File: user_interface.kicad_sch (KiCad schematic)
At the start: 29 parts, among them J3 Внутр. коннектор потенциометр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, J4 Внутр. коннектор галлетника (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, SW1 Кнопка тактовая 6x6 без фикса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, SW2 Кнопка тактовая 6x6 без фикса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, SW3 Кнопка тактовая 6x6 без фикса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, SW4 Кнопка тактовая 6x6 без фикса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, SW5 Кнопка тактовая 6x6 без фикса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, SW6 Кнопка тактовая 6x6 без фикса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

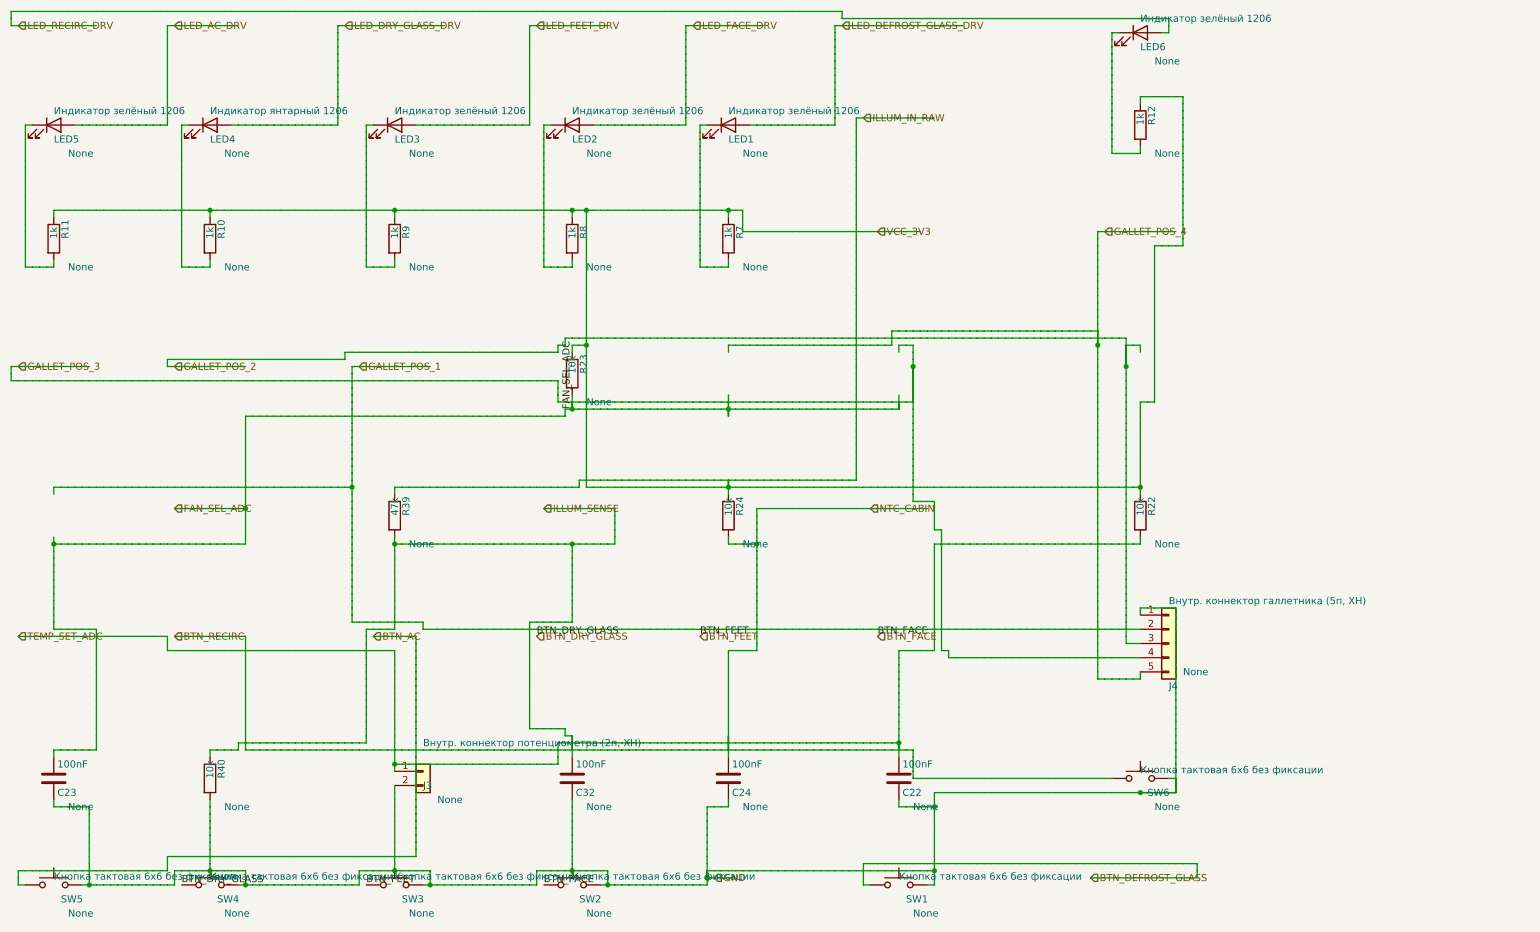
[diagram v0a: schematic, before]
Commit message: fix writer
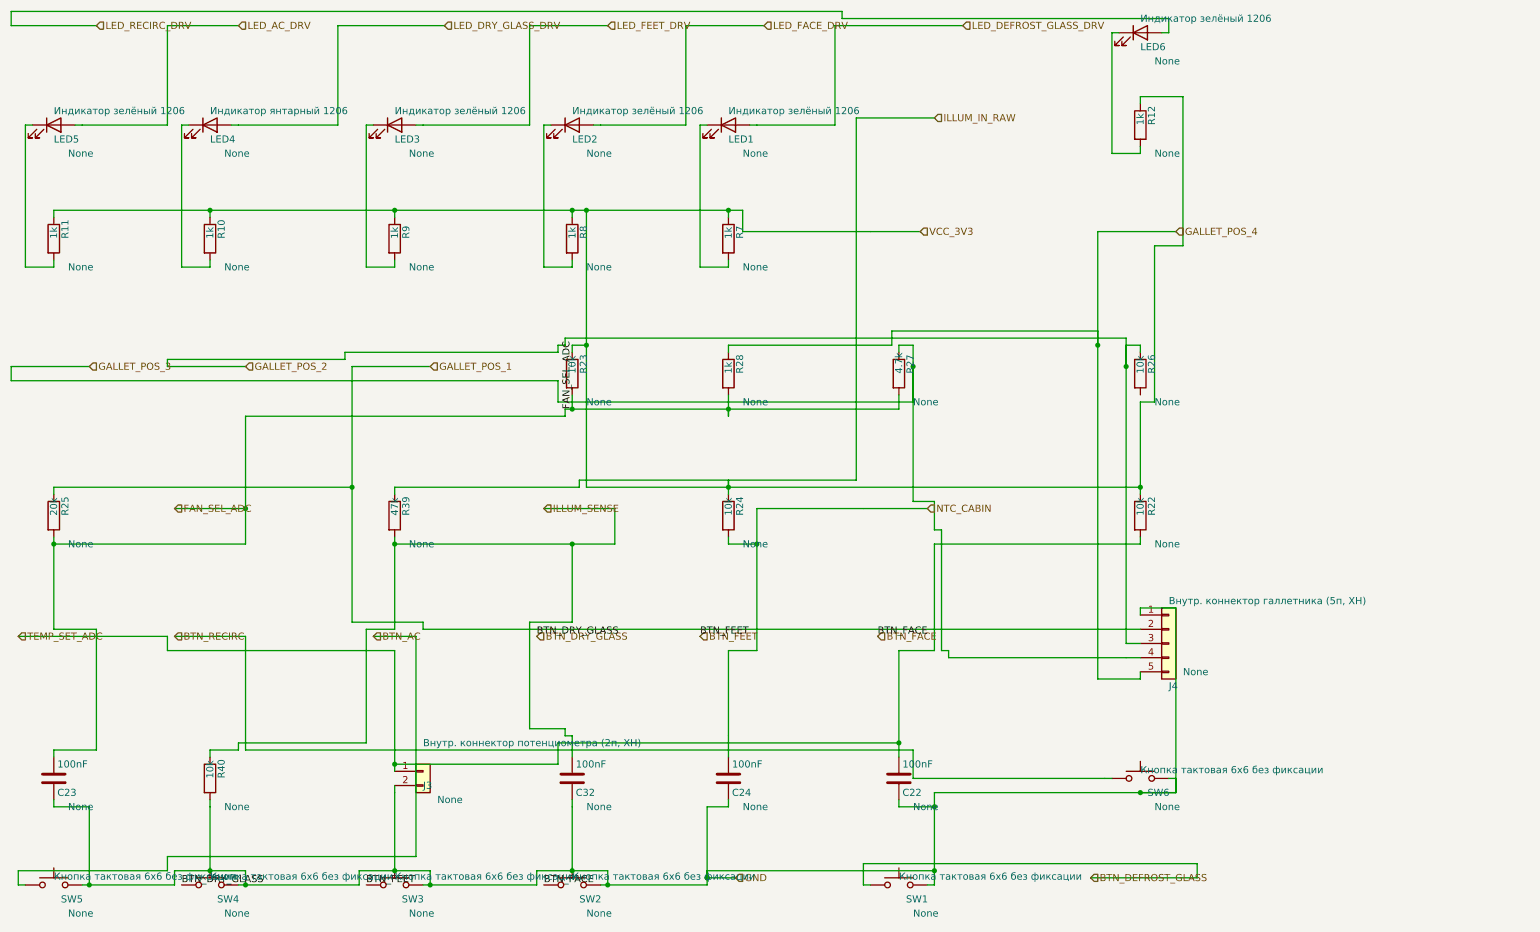
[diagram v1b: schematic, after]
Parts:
- added R25: 20k, symbol Device:R
- added R26: 10k, symbol Device:R
- added R27: 4.7k, symbol Device:R
- added R28: 1k, symbol Device:R
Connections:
- net BTN_AC: no longer C22.1, C22.2, C23.1, C23.2, C24.1, C24.2, C32.1, C32.2, J3.1 (Pin_1), J3.2 (Pin_2), J4.1 (Pin_1), J4.2 (Pin_2), J4.3 (Pin_3), J4.4 (Pin_4), J4.5 (Pin_5), LED1.1 (K), LED2.1 (K), LED3.1 (K), LED4.1 (K), R10.1, R10.2, R11.1, R12.1, R22.1, R22.2, R23.1, R23.2, R24.1, R24.2, R39.1, R39.2, R40.1, R40.2, R7.1, R7.2, R8.1, R8.2, R9.1, R9.2, SW1.1, SW1.2, SW2.2, SW3.2, SW4.2, SW5.2, SW6.1, SW6.2
- new net: LED3.1 (K), R9.2
- new net: LED1.1 (K), R7.2
- new net: LED2.1 (K), R8.2
- new net: LED4.1 (K), R10.2
- new net BTN_DEFROST_GLASS: SW1.1
- new net BTN_RECIRC: SW6.1
- new net FAN_SEL_ADC: C23.1, R23.2, R25.2, R27.2, R28.2
- new net GALLET_POS_1: J4.2 (Pin_2), R25.1
- new net GALLET_POS_2: J4.3 (Pin_3), R26.1
- new net GALLET_POS_3: J4.4 (Pin_4), R27.1
- new net GALLET_POS_4: J4.5 (Pin_5), R28.1
- new net GND: C22.2, C23.2, C24.2, C32.2, J3.2 (Pin_2), J4.1 (Pin_1), R40.2, SW1.2, SW2.2, SW3.2, SW4.2, SW5.2, SW6.2
- new net ILLUM_IN_RAW: R39.1
- new net ILLUM_SENSE: C32.1, R39.2, R40.1
- new net NTC_CABIN: C24.1, R24.2
- new net TEMP_SET_ADC: C22.1, J3.1 (Pin_1), R22.2
- new net VCC_3V3: R10.1, R11.1, R12.1, R22.1, R23.1, R24.1, R7.1, R8.1, R9.1
